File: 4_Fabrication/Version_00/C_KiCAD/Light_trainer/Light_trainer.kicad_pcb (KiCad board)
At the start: 2 copper layers, 105.2 x 105.2 mm, 25 parts, among them SW1 SW_Push, SW2 SW_Push, SW3 SW_Push, SW4 SW_Push, U1 LTC3525-5, U2 ESP32-DevKitC-32D

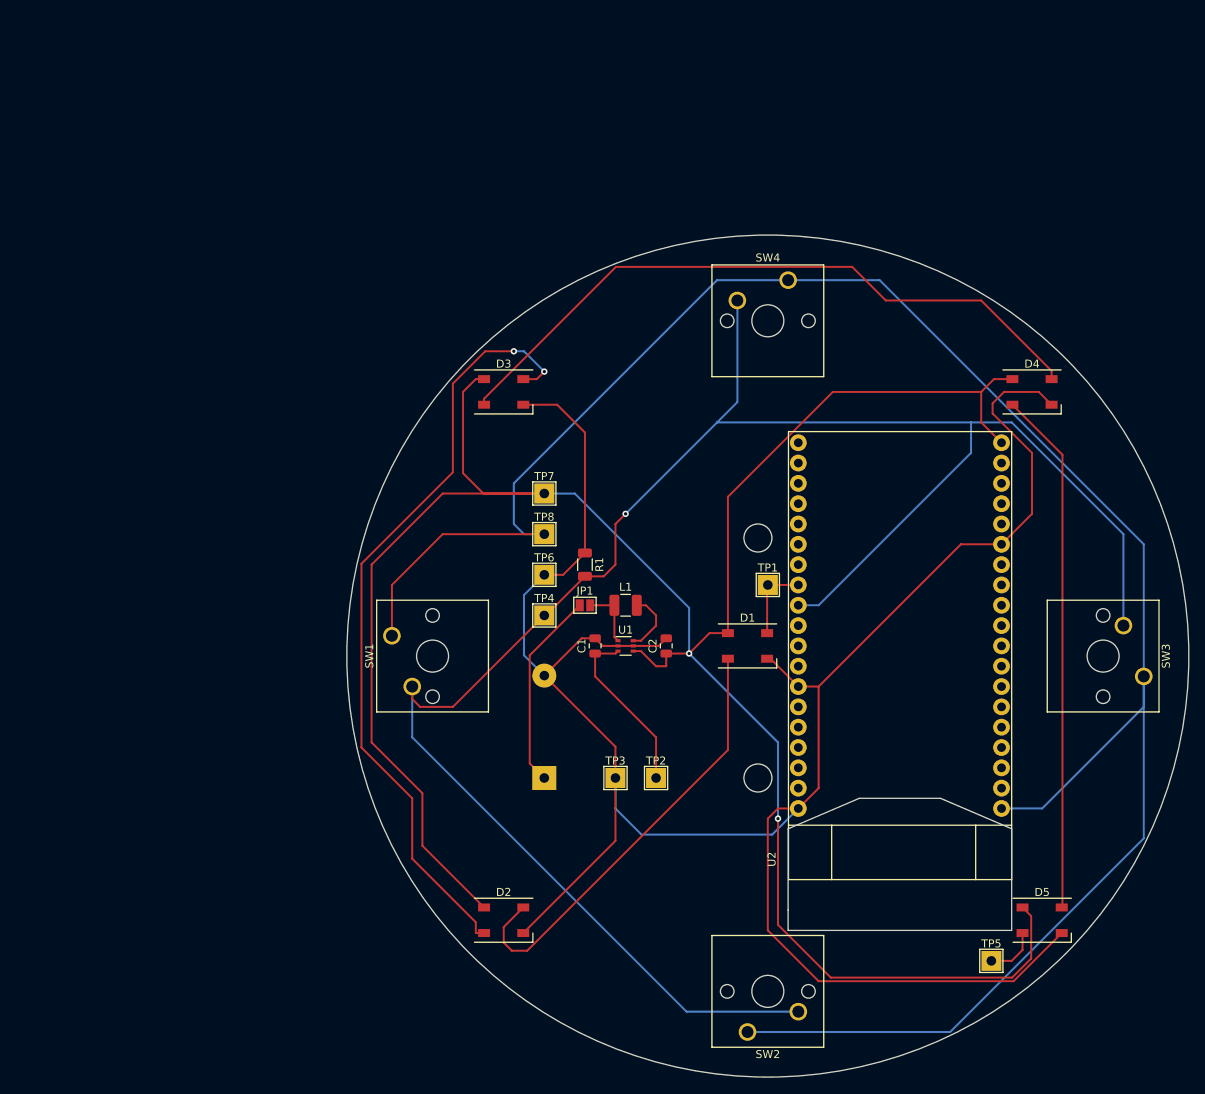
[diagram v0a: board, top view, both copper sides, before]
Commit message: placement + routage
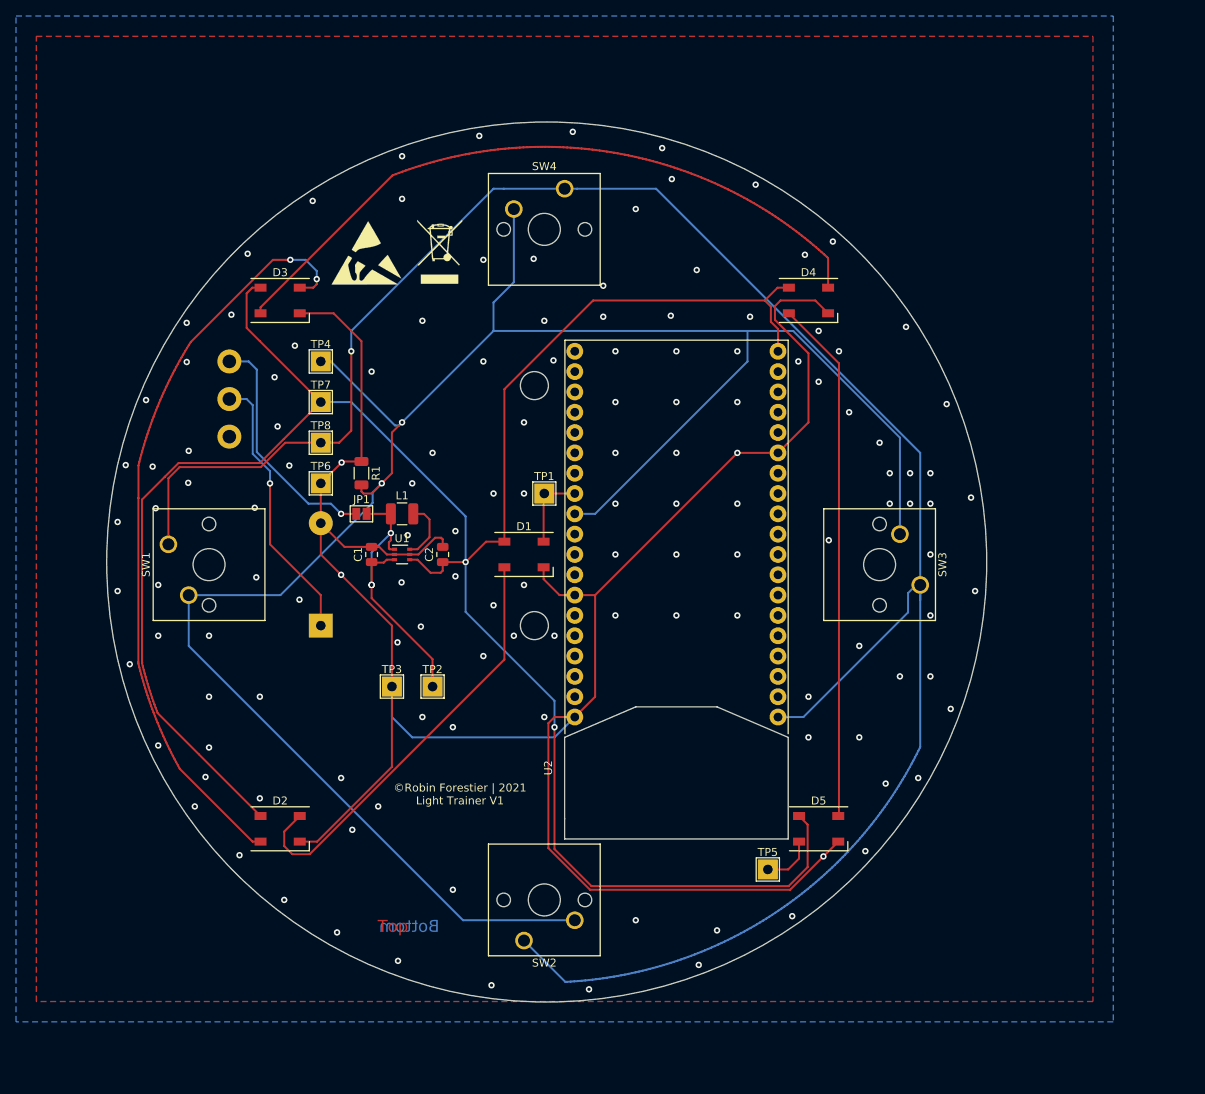
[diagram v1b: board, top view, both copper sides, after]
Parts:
- added REF**: WEEE-Logo_5.6x8mm_SilkScreen, Symbol:WEEE-Logo_5.6x8mm_SilkScreen, F.Cu at (126.6, 61.2)
- added REF**: ESD-Logo_8.9x8mm_SilkScreen, Symbol:ESD-Logo_8.9x8mm_SilkScreen, F.Cu at (117.5, 61.3)
- added SW5: SW_SPDT, Work_Forestier:C&K-1101M2S5CQE2, B.Cu at (100.3, 74.9)
- moved TP4 42.3 mm to (111.8, 74.9)
- moved BT1 33.8 mm to (111.8, 108.0)
- moved TP5 30.2 mm to (167.6, 138.4)
- moved C1 30.2 mm to (118.1, 99.1)
- moved L1 30.2 mm to (121.9, 94.0)
- moved SW1 30.2 mm to (92.7, 97.8)
- moved U1 30.2 mm to (121.9, 99.1)
- moved D2 30.2 mm to (106.7, 133.3)
- moved D5 30.2 mm to (174.0, 133.3)
- moved SW2 30.2 mm to (137.2, 147.3)
- moved TP1 30.2 mm to (139.7, 91.4)
- moved TP3 30.2 mm to (120.7, 115.6)
- moved C2 30.2 mm to (127.0, 99.1)
- moved D1 30.2 mm to (137.2, 99.1)
- moved D3 30.2 mm to (106.7, 67.3)
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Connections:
- JP1 pad 1: Net-(BT1-Pad1) -> Net-(JP1-Pad1)
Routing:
- net Net-(JP1-Pad1): track 0.00 -> 29.8 mm, vias 0 -> 1
- net switch: track 244.2 -> 259.9 mm, vias 1 -> 2
- net Net-(BT1-Pad1): track 24.9 -> 34.3 mm, vias 0 -> 1
- net Net-(C1-Pad1): track 29.3 -> 37.4 mm, vias 0 -> 3
- net +5V: track 290.4 -> 285.3 mm
- net Net-(D2-Pad4): track 97.5 -> 94.2 mm
- net +3V3: track 263.5 -> 266.0 mm, vias 0 -> 1
- net Net-(D1-Pad4): track 55.7 -> 54.1 mm
- net Net-(D3-Pad4): track 84.9 -> 86.2 mm
- net GND: track 277.5 -> 277.3 mm, vias 0 -> 136
- added copper zone on B.Cu, net GND
- added copper zone on F.Cu, net GND
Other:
- board size 105.2 x 105.2 mm -> 110 x 110 mm
- board text added: "AA"
- board text added: "Bottom"
- board text added: "ON - OFF"
- board text added: "Top"
- board text added: "©Robin Forestier | 2021 Light Trainer V1"
